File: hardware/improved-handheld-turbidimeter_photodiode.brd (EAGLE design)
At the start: 23 x 17.8 mm, 13 parts

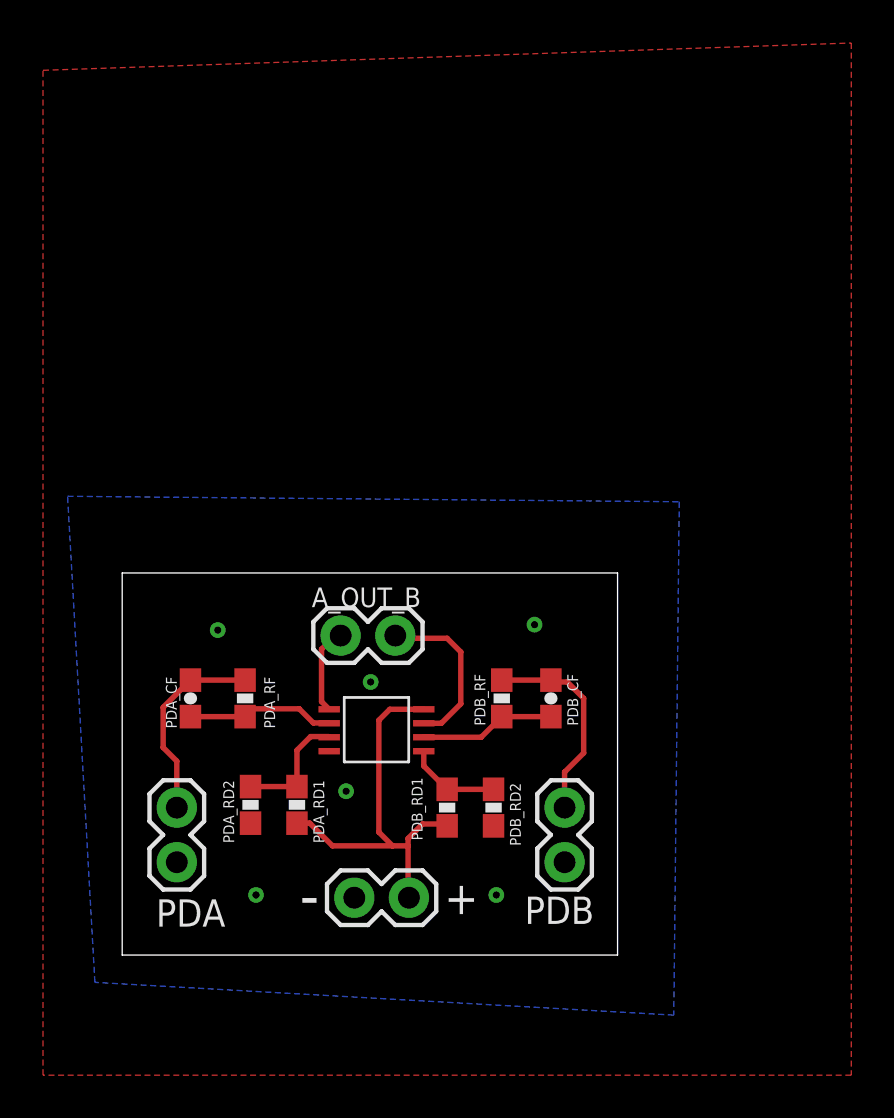
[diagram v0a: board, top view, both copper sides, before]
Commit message: upd
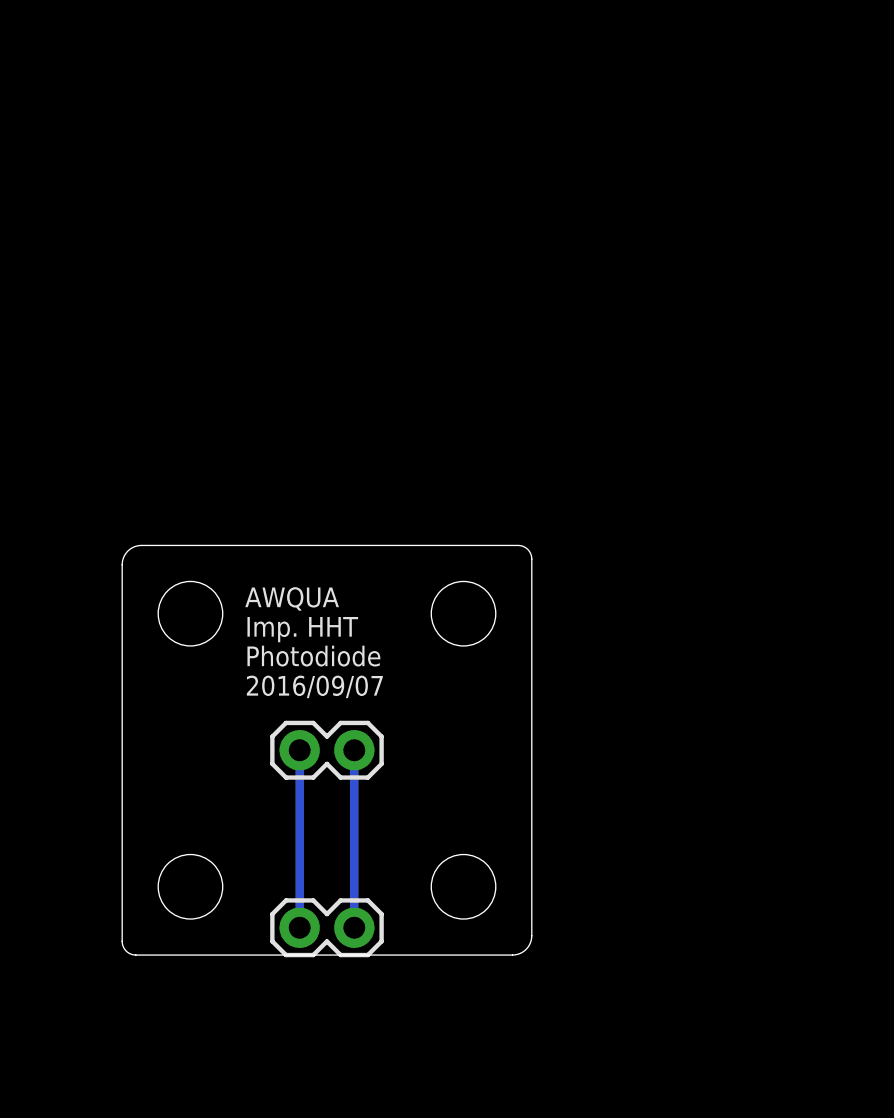
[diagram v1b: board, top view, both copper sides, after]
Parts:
- removed A_OUT_B, JP3, PDA, PDB: (no value), SparkFun-Connectors:1X02
- removed PDA_CF, PDB_CF: (no value), SparkFun-Passives:0603-CAP
- removed PDA_RD1, PDA_RD2, PDA_RF, PDB_RD1, PDB_RD2, PDB_RF: (no value), SparkFun-Passives:0603-RES
- removed U$2: ADA4528-2, awqua_eagle_library:ADA4528-2
- added J1, J2: (no value), SparkFun-Connectors:1X02
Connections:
- removed net GND: JP3.2, PDA.2, PDA_RD2.1, PDB.1, PDB_RD2.1, U$2.P$4
- removed net N$3: PDB.2, PDB_CF.2, PDB_RF.1
- removed net N$4: PDB_CF.1, PDB_RF.2, U$2.P$6
- removed net N$5: PDA_RD1.2, PDA_RD2.2, U$2.P$3
- removed net N$6: PDB_RD1.2, PDB_RD2.2, U$2.P$5
- removed net OUTA: A_OUT_B.1, U$2.P$1
- removed net OUTB: A_OUT_B.2, U$2.P$7
- removed net VCC: JP3.1, PDA_RD1.1, PDB_RD1.1, U$2.P$8
- net N$1: now also J1.2, J2.1; no longer PDA.1, PDA_CF.2, PDA_RF.1
- net N$2: now also J1.1, J2.2; no longer PDA_CF.1, PDA_RF.2, U$2.P$2
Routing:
- net VCC: track 18.9 -> 0.00 mm
- net N$3: track 9.61 -> 0.00 mm
- net OUTB: track 7.87 -> 0.00 mm
- net N$4: track 6.82 -> 0.00 mm
- net N$5: track 5.62 -> 0.00 mm
- net N$6: track 4.38 -> 0.00 mm
- net OUTA: track 4.09 -> 0.00 mm
- net N$2: track 6.88 -> 8.26 mm
- net N$1: track 9.26 -> 8.26 mm
- removed copper zone on layer 1, net GND
- removed copper zone on layer 16, net GND
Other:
- board size 23 x 17.8 mm -> 19.1 x 19.1 mm
- board text added: "AWQUA Imp. HHT Photodiode 2016/09/07"
- board text removed: "+"
- board text removed: "-"
- board text removed: "AWQUA TIA Board v1.0 2016/08/24"
